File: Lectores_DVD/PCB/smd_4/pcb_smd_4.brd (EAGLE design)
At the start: 20.8 x 22.8 mm, 2 parts, among them J1 52793-0470

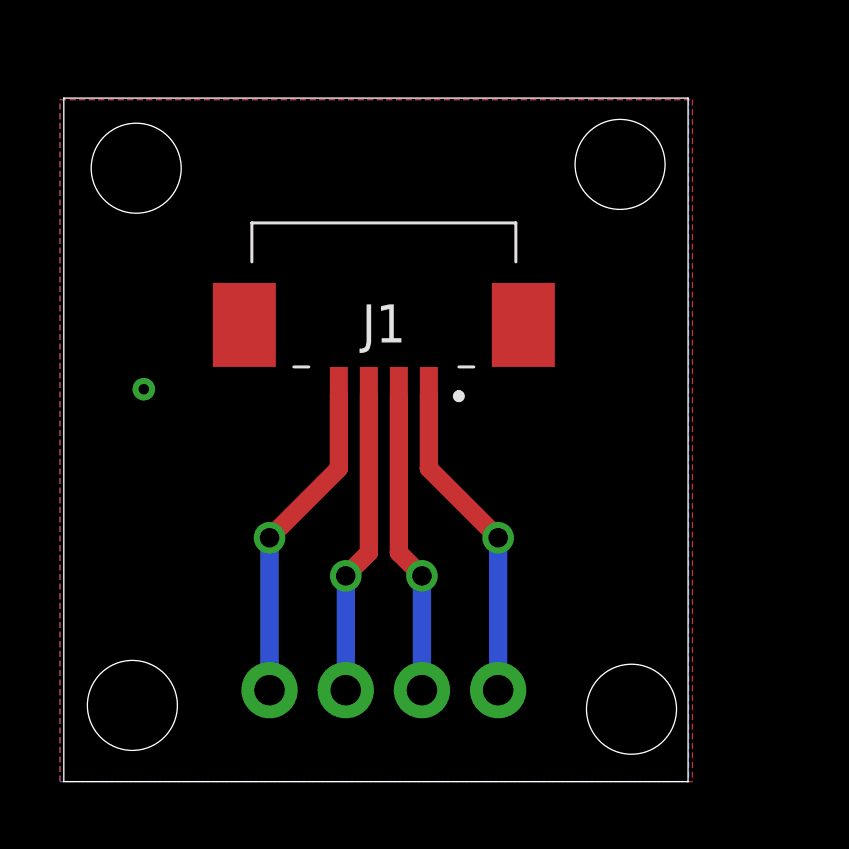
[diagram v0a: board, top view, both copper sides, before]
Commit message: Actualizacion
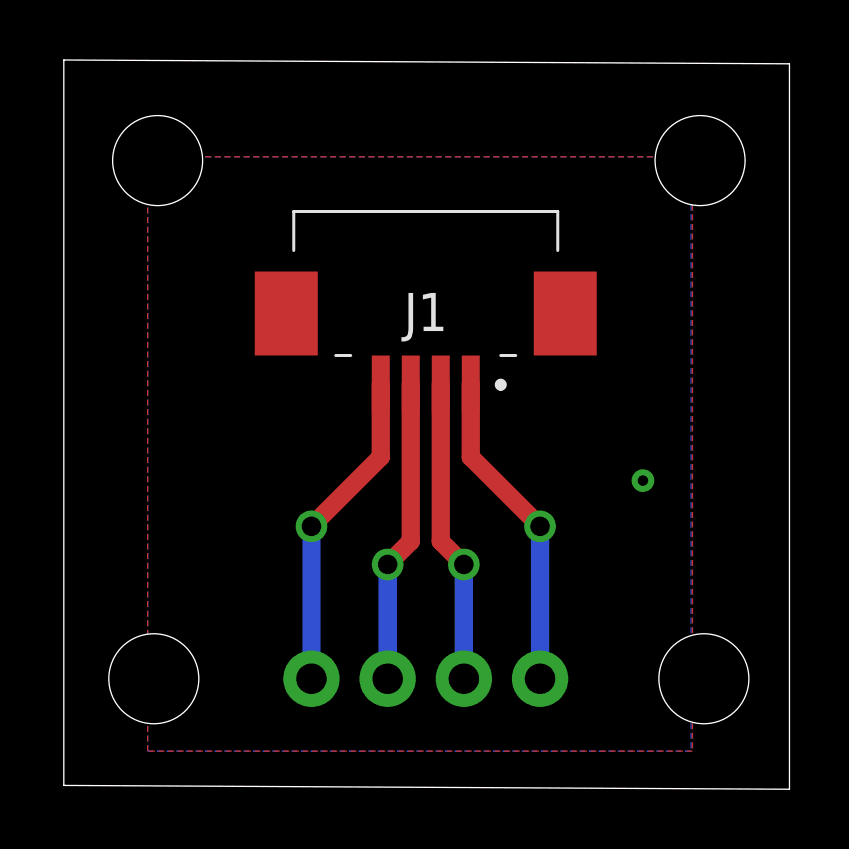
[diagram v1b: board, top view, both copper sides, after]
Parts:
- moved J1 1.45 mm to (14.1, 16.9)
- moved J2 1.45 mm to (17.9, 4.19)
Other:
- board size 20.8 x 22.8 mm -> 24.2 x 24.3 mm
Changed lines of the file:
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@@
 <setting verticaltext="up"/>
 </settings>
-<grid distance="1.27" unitdist="mm" unit="mm" style="lines" multiple="1" display="no" altdistance="5" altunitdist="mil" altunit="mm"/>
+<grid distance="0.127" unitdist="mm" unit="mm" style="lines" multiple="1" display="no" altdistance="5" altunitdist="mil" altunit="mm"/>
 <layers>
 <layer number="1" name="Top" color="4" fill="1" visible="yes" active="yes"/>
@@
 <board>
 <plain>
-<wire x1="2.032" y1="0.762" x2="22.84" y2="0.762" width="0" layer="20"/>
-<wire x1="22.84" y1="0.762" x2="22.84" y2="23.546" width="0" layer="20"/>
-<wire x1="22.84" y1="23.546" x2="2.032" y2="23.546" width="0" layer="20"/>
-<wire x1="2.032" y1="23.546" x2="2.032" y2="0.762" width="0" layer="20"/>
-<hole x="4.445" y="21.209" drill="3"/>
-<hole x="20.574" y="21.336" drill="3"/>
-<hole x="20.955" y="3.175" drill="3"/>
-<hole x="4.318" y="3.302" drill="3"/>
+<wire x1="2.032" y1="0.635" x2="26.221" y2="0.508" width="0" layer="20"/>
+<wire x1="26.221" y1="0.508" x2="26.221" y2="24.689" width="0" layer="20"/>
+<wire x1="26.221" y1="24.689" x2="2.032" y2="24.816" width="0" layer="20"/>
+<wire x1="2.032" y1="24.816" x2="2.032" y2="0.635" width="0" layer="20"/>
+<hole x="5.159" y="21.463" drill="3"/>
+<hole x="23.241" y="21.463" drill="3"/>
+<hole x="5.032" y="4.191" drill="3"/>
+<hole x="23.368" y="4.191" drill="3"/>
 </plain>
 <attributes>
@@
 </autorouter>
 <elements>
-<element name="J1" library="52793-0470" package="527930472" value="52793-0470" x="12.7" y="16.51" smashed="yes" rot="R180">
-<attribute name="ALLIED_NUMBER" value="71463721" x="-6.35" y="20.32" size="1.778" layer="27" rot="R180" display="off"/>
-<attribute name="ALLIED_PRICE-STOCK" value="https://www.alliedelec.com/molexincorporated-52793-0470/71463721/" x="-6.35" y="20.32" size="1.778" layer="27" rot="R180" display="off"/>
-<attribute name="DESCRIPTION" value="Molex 52793 Series 1mm Pitch 4 Way SMT Female FPC Connector, Non-ZIF" x="-6.35" y="20.32" size="1.778" layer="27" rot="R180" display="off"/>
-<attribute name="HEIGHT" value="3.1mm" x="-6.35" y="20.32" size="1.778" layer="27" rot="R180" display="off"/>
-<attribute name="MANUFACTURER_NAME" value="Molex" x="-6.35" y="20.32" size="1.778" layer="27" rot="R180" display="off"/>
-<attribute name="MANUFACTURER_PART_NUMBER" value="52793-0470" x="-6.35" y="20.32" size="1.778" layer="27" rot="R180" display="off"/>
-<attribute name="MOUSER_PART_NUMBER" value="538-52793-0470" x="-6.35" y="20.32" size="1.778" layer="27" rot="R180" display="off"/>
-<attribute name="MOUSER_PRICE-STOCK" value="https://www.mouser.com/Search/Refine.aspx?Keyword=538-52793-0470" x="-6.35" y="20.32" size="1.778" layer="27" rot="R180" display="off"/>
-<attribute name="NAME" x="12.7" y="16.035" size="1.27" layer="25" rot="R180" align="center"/>
-<attribute name="RS_PART_NUMBER" value="1791963" x="-6.35" y="20.32" size="1.778" layer="27" rot="R180" display="off"/>
-<attribute name="RS_PRICE-STOCK" value="http://uk.rs-online.com/web/p/products/1791963" x="-6.35" y="20.32" size="1.778" layer="27" rot="R180" display="off"/>
-<attribute name="VALUE" x="12.7" y="16.035" size="1.27" layer="27" rot="R180" align="center"/>
+<element name="J1" library="52793-0470" package="527930472" value="52793-0470" x="14.097" y="16.891" smashed="yes" rot="R180">
+<attribute name="ALLIED_NUMBER" value="71463721" x="-4.953" y="20.701" size="1.778" layer="27" rot="R180" display="off"/>
+<attribute name="ALLIED_PRICE-STOCK" value="https://www.alliedelec.com/molexincorporated-52793-0470/71463721/" x="-4.953" y="20.701" size="1.778" layer="27" rot="R180" display="off"/>
+<attribute name="DESCRIPTION" value="Molex 52793 Series 1mm Pitch 4 Way SMT Female FPC Connector, Non-ZIF" x="-4.953" y="20.701" size="1.778" layer="27" rot="R180" display="off"/>
+<attribute name="HEIGHT" value="3.1mm" x="-4.953" y="20.701" size="1.778" layer="27" rot="R180" display="off"/>
+<attribute name="MANUFACTURER_NAME" value="Molex" x="-4.953" y="20.701" size="1.778" layer="27" rot="R180" display="off"/>
+<attribute name="MANUFACTURER_PART_NUMBER" value="52793-0470" x="-4.953" y="20.701" size="1.778" layer="27" rot="R180" display="off"/>
+<attribute name="MOUSER_PART_NUMBER" value="538-52793-0470" x="-4.953" y="20.701" size="1.778" layer="27" rot="R180" display="off"/>
+<attribute name="MOUSER_PRICE-STOCK" value="https://www.mouser.com/Search/Refine.aspx?Keyword=538-52793-0470" x="-4.953" y="20.701" size="1.778" layer="27" rot="R180" display="off"/>
+<attribute name="NAME" x="14.097" y="16.416" size="1.27" layer="25" rot="R180" align="center"/>
+<attribute name="RS_PART_NUMBER" value="1791963" x="-4.953" y="20.701" size="1.778" layer="27" rot="R180" display="off"/>
+<attribute name="RS_PRICE-STOCK" value="http://uk.rs-online.com/web/p/products/1791963" x="-4.953" y="20.701" size="1.778" layer="27" rot="R180" display="off"/>
+<attribute name="VALUE" x="14.097" y="16.416" size="1.27" layer="27" rot="R180" align="center"/>
 </element>
-<element name="J2" library="SparkFun-Connectors" package="1X04" value="" x="16.51" y="3.81" smashed="yes" rot="MR0">
-<attribute name="NAME" x="17.78" y="5.207" size="0.6096" layer="26" font="vector" ratio="20" rot="MR0"/>
-<attribute name="PROD_ID" value="CONN-09696" x="-6.35" y="-6.35" size="1.778" layer="28" rot="MR0" display="off"/>
-<attribute name="VALUE" x="17.78" y="1.778" size="0.6096" layer="28" font="vector" ratio="20" rot="MR0"/>
+<element name="J2" library="SparkFun-Connectors" package="1X04" value="" x="17.907" y="4.191" smashed="yes" rot="MR0">
+<attribute name="NAME" x="19.177" y="5.588" size="0.6096" layer="26" font="vector" ratio="20" rot="MR0"/>
+<attribute name="PROD_ID" value="CONN-09696" x="-4.953" y="-5.969" size="1.778" layer="28" rot="MR0" display="off"/>
+<attribute name="VALUE" x="19.177" y="2.159" size="0.6096" layer="28" font="vector" ratio="20" rot="MR0"/>
 </element>
 </elements>
@@
 <contactref element="J1" pad="3"/>
 <contactref element="J2" pad="3"/>
-<wire x1="12.2" y1="13.635" x2="12.2" y2="8.39" width="0.6096" layer="1"/>
-<wire x1="12.2" y1="8.39" x2="11.43" y2="7.62" width="0.6096" layer="1"/>
-<via x="11.43" y="7.62" extent="1-16" drill="0.65"/>
-<wire x1="11.43" y1="7.62" x2="11.43" y2="3.81" width="0.6096" layer="16"/>
+<wire x1="13.597" y1="14.016" x2="13.597" y2="8.771" width="0.6096" layer="1"/>
+<wire x1="13.597" y1="8.771" x2="12.827" y2="8.001" width="0.6096" layer="1"/>
+<via x="12.827" y="8.001" extent="1-16" drill="0.65"/>
+<wire x1="12.827" y1="8.001" x2="12.827" y2="4.191" width="0.6096" layer="16"/>
 </signal>
 <signal name="N$5">
 <contactref element="J1" pad="1"/>
 <contactref element="J2" pad="1"/>
-<wire x1="14.2" y1="13.635" x2="14.2" y2="11.2" width="0.6096" layer="1"/>
-<wire x1="14.2" y1="11.2" x2="16.51" y2="8.89" width="0.6096" layer="1"/>
-<via x="16.51" y="8.89" extent="1-16" drill="0.65"/>
-<wire x1="16.51" y1="8.89" x2="16.51" y2="3.81" width="0.6096" layer="16"/>
+<wire x1="15.597" y1="14.016" x2="15.597" y2="11.581" width="0.6096" layer="1"/>
+<wire x1="15.597" y1="11.581" x2="17.907" y2="9.271" width="0.6096" layer="1"/>
+<via x="17.907" y="9.271" extent="1-16" drill="0.65"/>
+<wire x1="17.907" y1="9.271" x2="17.907" y2="4.191" width="0.6096" layer="16"/>
 </signal>
 <signal name="N$1">
 <contactref element="J2" pad="2"/>
 <contactref element="J1" pad="2"/>
-<wire x1="13.2" y1="13.635" x2="13.2" y2="8.39" width="0.6096" layer="1"/>
-<wire x1="13.2" y1="8.39" x2="13.97" y2="7.62" width="0.6096" layer="1"/>
-<via x="13.97" y="7.62" extent="1-16" drill="0.65"/>
-<wire x1="13.97" y1="7.62" x2="13.97" y2="3.81" width="0.6096" layer="16"/>
+<wire x1="14.597" y1="14.016" x2="14.597" y2="8.771" width="0.6096" layer="1"/>
+<wire x1="14.597" y1="8.771" x2="15.367" y2="8.001" width="0.6096" layer="1"/>
+<via x="15.367" y="8.001" extent="1-16" drill="0.65"/>
+<wire x1="15.367" y1="8.001" x2="15.367" y2="4.191" width="0.6096" layer="16"/>
 </signal>
 <signal name="N$3">
 <contactref element="J2" pad="4"/>
 <contactref element="J1" pad="4"/>
-<wire x1="11.2" y1="13.635" x2="11.2" y2="11.2" width="0.6096" layer="1"/>
-<wire x1="11.2" y1="11.2" x2="8.89" y2="8.89" width="0.6096" layer="1"/>
-<via x="8.89" y="8.89" extent="1-16" drill="0.65"/>
-<wire x1="8.89" y1="8.89" x2="8.89" y2="3.81" width="0.6096" layer="16"/>
+<wire x1="12.597" y1="14.016" x2="12.597" y2="11.581" width="0.6096" layer="1"/>
+<wire x1="12.597" y1="11.581" x2="10.287" y2="9.271" width="0.6096" layer="1"/>
+<via x="10.287" y="9.271" extent="1-16" drill="0.65"/>
+<wire x1="10.287" y1="9.271" x2="10.287" y2="4.191" width="0.6096" layer="16"/>
 </signal>
 <signal name="GND">
 <polygon width="0.1524" layer="1">
-<vertex x="1.905" y="23.495"/>
-<vertex x="22.987" y="23.495"/>
-<vertex x="22.987" y="0.762"/>
-<vertex x="1.905" y="0.762"/>
+<vertex x="4.826" y="21.59"/>
+<vertex x="22.987" y="21.59"/>
+<vertex x="22.987" y="1.778"/>
+<vertex x="4.826" y="1.778"/>
 </polygon>
 <polygon width="0.1524" layer="16">
-<vertex x="1.905" y="23.495"/>
-<vertex x="22.86" y="23.495"/>
-<vertex x="22.86" y="0.762"/>
-<vertex x="1.905" y="0.762"/>
+<vertex x="4.826" y="21.59"/>
+<vertex x="22.939" y="21.59"/>
+<vertex x="22.939" y="1.778"/>
+<vertex x="4.826" y="1.778"/>
 </polygon>
-<via x="4.699" y="13.843" extent="1-16" drill="0.35"/>
+<via x="21.336" y="10.795" extent="1-16" drill="0.35"/>
 </signal>
 </signals>
